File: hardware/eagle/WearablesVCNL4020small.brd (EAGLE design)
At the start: 11.5 x 12 mm, 11 parts

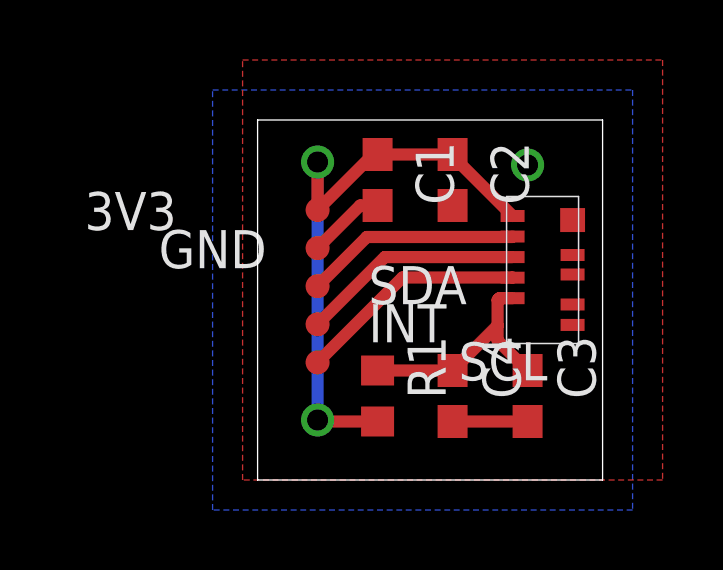
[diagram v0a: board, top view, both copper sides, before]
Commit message: updated schematics and board files.
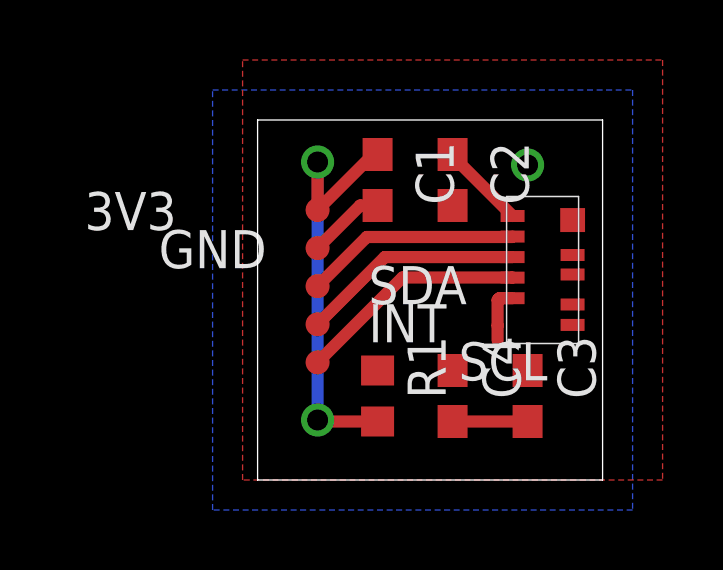
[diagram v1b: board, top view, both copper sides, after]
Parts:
- R1: value 10 -> 10R
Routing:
- net VDD: track 7.91 -> 1.87 mm
- net +3V3: track 20.4 -> 17.8 mm
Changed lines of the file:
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@@
 <?xml version="1.0" encoding="utf-8"?>
 <!DOCTYPE eagle SYSTEM "eagle.dtd">
-<eagle version="7.6.0">
+<eagle version="7.5.0">
 <drawing>
 <settings>
@@
 <attribute name="NAME" x="6" y="9.8" size="1.27" layer="25" rot="R270"/>
 </element>
-<element name="R1" library="resistor" package="R0603" value="10" x="2.5" y="7.8" smashed="yes" rot="R270">
+<element name="R1" library="resistor" package="R0603" value="10R" x="2.5" y="7.8" smashed="yes" rot="R270">
 <attribute name="NAME" x="3.5" y="9.8" size="1.27" layer="25" rot="R270"/>
 </element>
@@
 <wire x1="6.56" y1="11.06" x2="6.5" y2="11" width="0.4064" layer="1"/>
 <wire x1="6.5" y1="11" x2="6.5" y2="10.15" width="0.4064" layer="1"/>
-<wire x1="6.5" y1="10.15" x2="5" y2="8.65" width="0.4064" layer="1"/>
 <wire x1="6.5" y1="10.15" x2="6.5" y2="9.65" width="0.4064" layer="1"/>
-<wire x1="6.5" y1="9.65" x2="7.5" y2="8.65" width="0.4064" layer="1"/>
-<wire x1="2.5" y1="8.65" x2="5" y2="8.65" width="0.4064" layer="1"/>
+<wire x1="6.5" y1="9.65" x2="7.5" y2="8.65" width="0" layer="19" extent="1-1"/>
+<wire x1="5" y1="8.65" x2="6.5" y2="9.65" width="0" layer="19" extent="1-1"/>
+<wire x1="2.5" y1="8.65" x2="5" y2="8.65" width="0" layer="19" extent="1-1"/>
 </signal>
 <signal name="+3V3">
 <contactref element="R1" pad="2"/>
-<contactref element="C2" pad="1"/>
 <contactref element="C1" pad="1"/>
 <contactref element="U$1" pad="ANODE_EM"/>
 <contactref element="3V3" pad="TP"/>
-<wire x1="2.5" y1="15.85" x2="5" y2="15.85" width="0.4064" layer="1"/>
-<wire x1="5" y1="15.85" x2="5" y2="15.8" width="0.4064" layer="1"/>
 <wire x1="5" y1="15.8" x2="7" y2="13.8" width="0.4064" layer="1"/>
 <wire x1="2.5" y1="6.95" x2="0.55" y2="6.95" width="0.4064" layer="1"/>
@@
 <via x="0.5" y="15.6" extent="1-16" drill="0.7" diameter="0.8128"/>
 <wire x1="0.5" y1="15.6" x2="0.5" y2="14" width="0.4064" layer="1"/>
+<contactref element="C2" pad="1"/>
+<wire x1="5" y1="15.85" x2="5" y2="15.8" width="0" layer="19" extent="1-1"/>
+<wire x1="2.5" y1="15.85" x2="5" y2="15.8" width="0" layer="19" extent="1-1"/>
 </signal>
 <signal name="SDA">
